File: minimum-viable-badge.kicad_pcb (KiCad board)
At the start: 2 copper layers, 120 x 64 mm, 67 parts, among them J101 EDGE_CONNECTOR, P101 USB, P102 BATTERY, P103 POT_LONG, P104 BUTTON_A, P105 BUTTON_B, P106 POT_SHORT, P107 MECH, P108 MECH, P109 MECH, P301 eInk, Q101 S8050, Q102 S8050, Q201 FDN340P, Q301 IRLML0030TRPBF, SW101 PRGM, SW102 RESET, SW201 ON|OFF, U101 ESP32-WROOM, U102 CP2102, U201 MCP73831, U202 NCP5501

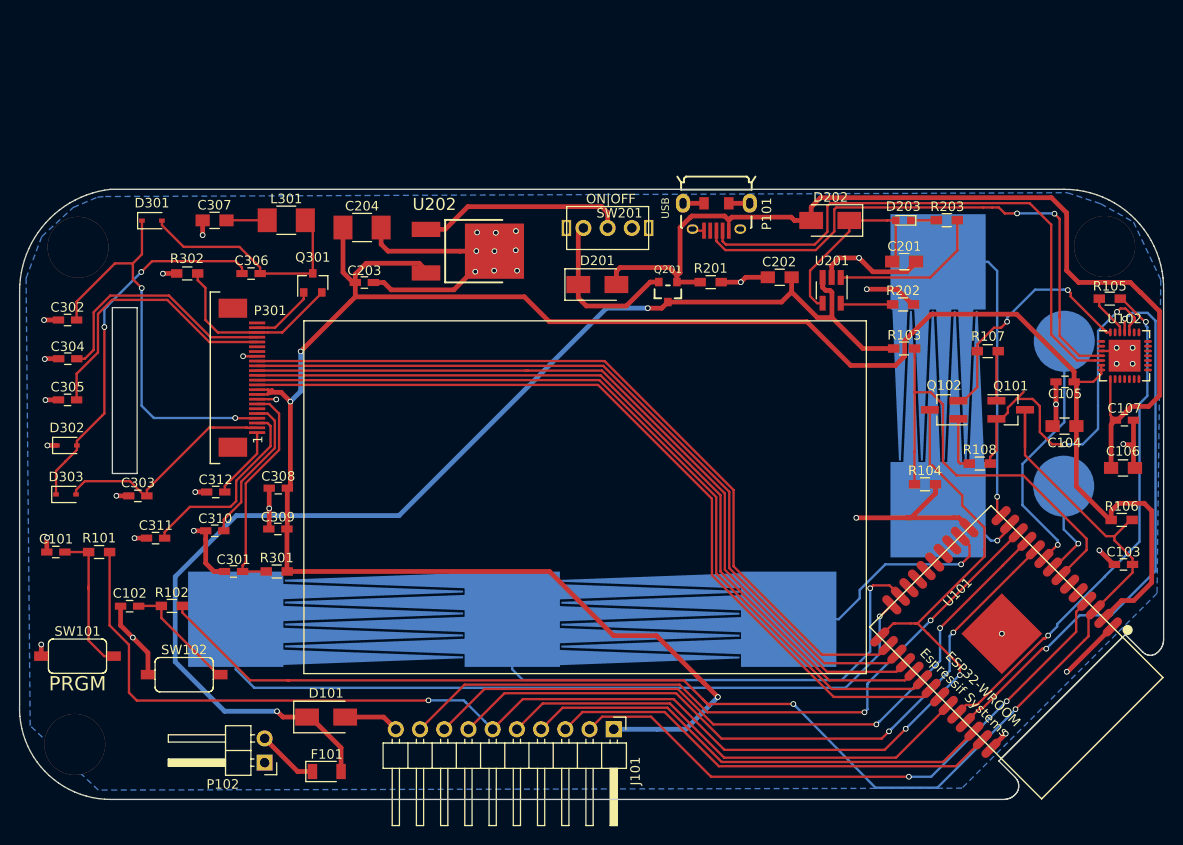
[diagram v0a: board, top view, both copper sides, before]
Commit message: Flipped is better.
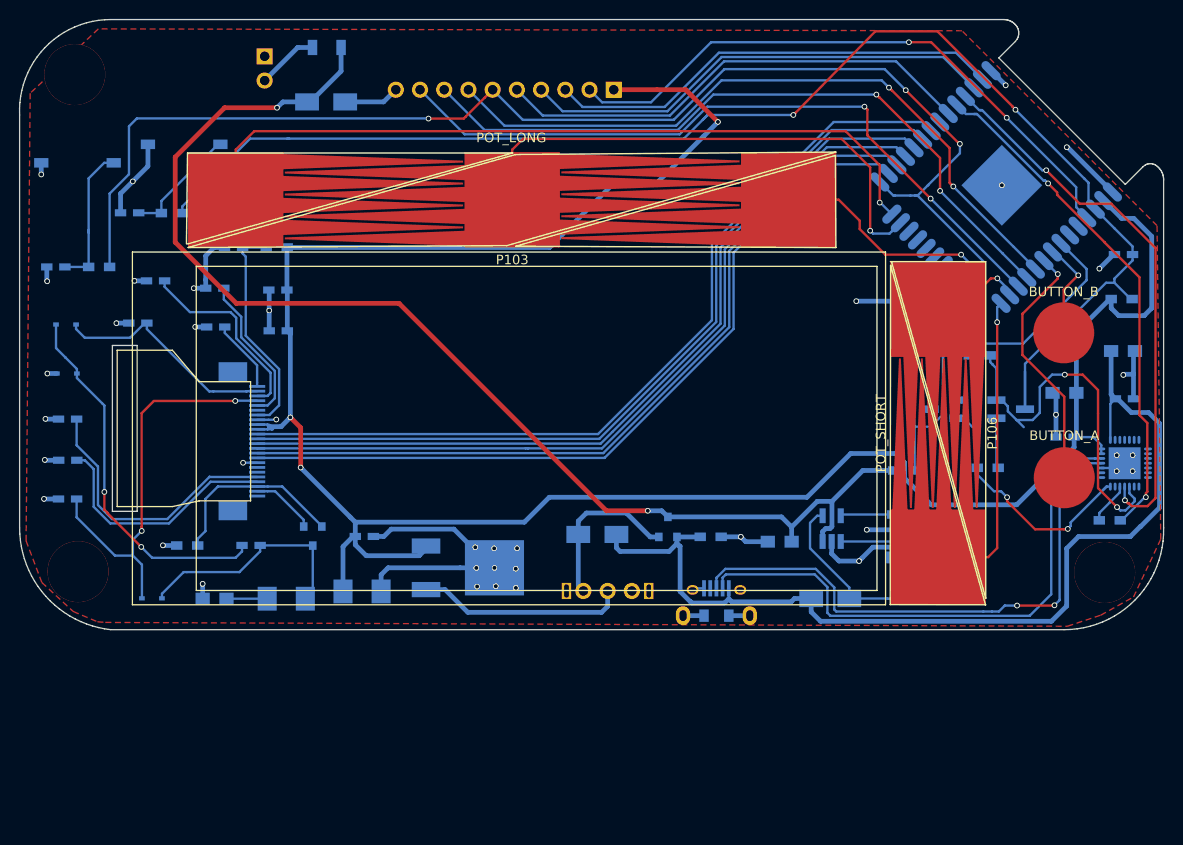
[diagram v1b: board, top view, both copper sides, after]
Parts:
- C101, C102, C103, C104, C105, C106, C107, C201, C202, C203, C204, C301, C302, C303, C304, C305, C306, C307, C308, C309, C310, C311, C312, D101, D201, D202, D203, D301, D302, D303, F101, J101, L301, P101, P102, P107, P108, P109, P301, Q101, Q102, Q201, Q301, R101, R102, R103, R104, R105, R106, R107, R108, R201, R202, R203, R301, R302, SW101, SW102, SW201, U101, U102, U201, U202: moved to B.Cu
- P103, P104, P105, P106: moved to F.Cu
- moved F101 75.9 mm to (52.2, 21.1)
- moved P102 74.1 mm to (45.7, 22.1)
- moved P108 70.3 mm to (25.8, 24.0)
- moved J101 67.1 mm to (82.3, 25.6), turned to 90 degrees
- moved D101 64.5 mm to (52.1, 26.8)
- moved SW102 55.6 mm to (37.3, 31.3)
- moved SW101 51.7 mm to (26.1, 33.2)
- moved U101 50.9 mm to (124.5, 33.6), turned to 315 degrees
- moved P103 44.0 mm to (71.7, 37.1)
- moved C102 41.3 mm to (31.5, 38.5)
- moved R102 41.2 mm to (36.0, 38.5)
- moved P101 41.1 mm to (93.0, 79.6), turned to 90 degrees
- moved R203 39.7 mm to (117.3, 79.0)
- moved L301 39.7 mm to (48.0, 78.9)
- moved C307 39.7 mm to (40.5, 78.9)
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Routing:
- added copper zone on F.Cu, net GND
- removed copper zone on B.Cu, net GND
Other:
- outline, holes or cut-outs redrawn
